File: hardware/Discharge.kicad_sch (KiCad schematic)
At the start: 6 parts

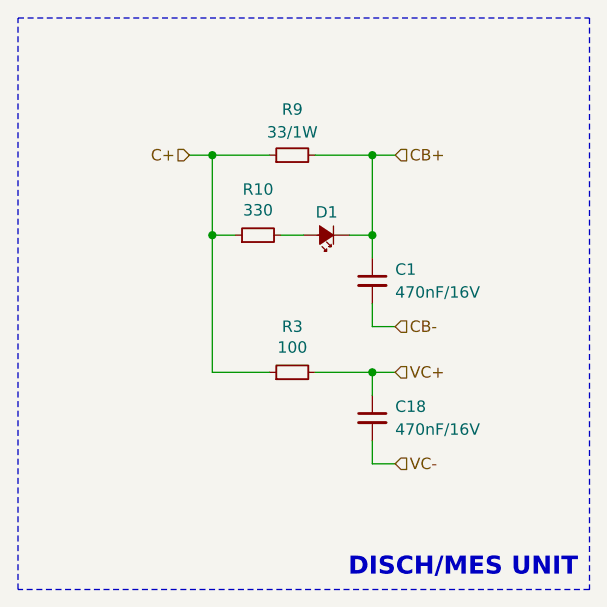
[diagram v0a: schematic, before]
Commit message: dev-hard-v3.0
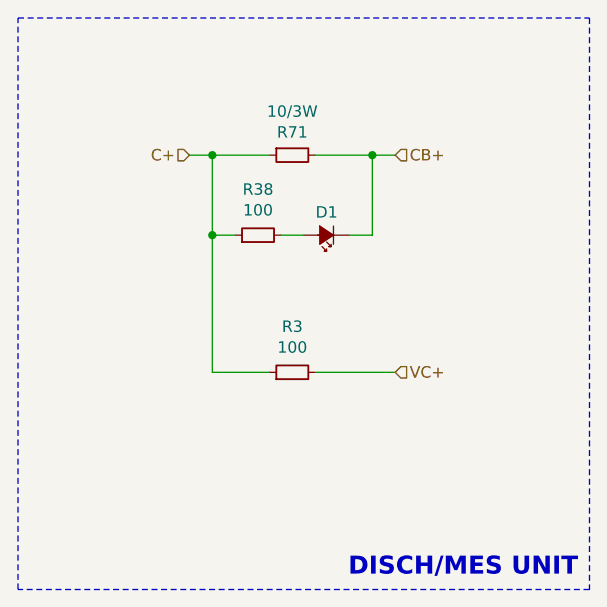
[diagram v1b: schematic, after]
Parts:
- removed C1, C18: 470nF/16V, Capacitor_SMD:C_0603_1608Metric, symbol Device:C_Small
- removed R10: 330, Resistor_SMD:R_0603_1608Metric, symbol PUTM_EV_BMS_HV_Slave_2021-rescue:R_Small-Device
- removed R9: 33/1W, Resistor_SMD:R_1206_3216Metric, symbol PUTM_EV_BMS_HV_Slave_2021-rescue:R_Small-Device
- added R38: 100, Resistor_SMD:R_0603_1608Metric, symbol PUTM_EV_BMS_HV_Slave_2021-rescue:R_Small-Device
- added R71: 10/3W, Resistor_SMD:R_2512_6332Metric, symbol PUTM_EV_BMS_HV_Slave_2021-rescue:R_Small-Device
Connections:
- net C+: now also R38.1, R71.1
- net CB+: now also R71.2
- net at D1.2 (A): now also R38.2
